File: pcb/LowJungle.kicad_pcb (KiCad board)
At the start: 2 copper layers, 378.6 x 152.4 mm, 255 parts

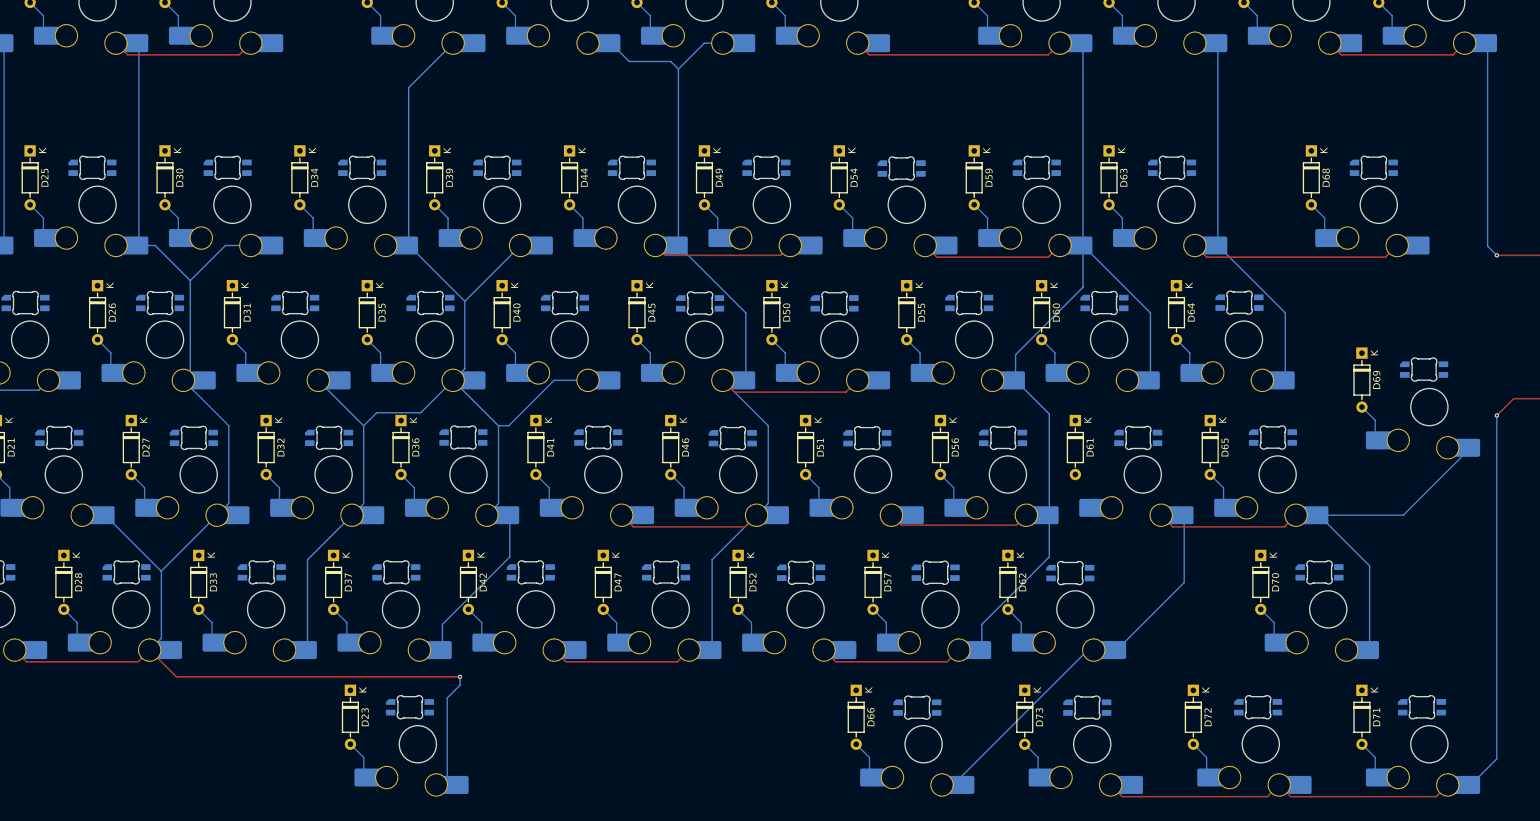
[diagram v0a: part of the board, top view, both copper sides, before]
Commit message: Added stabilizers
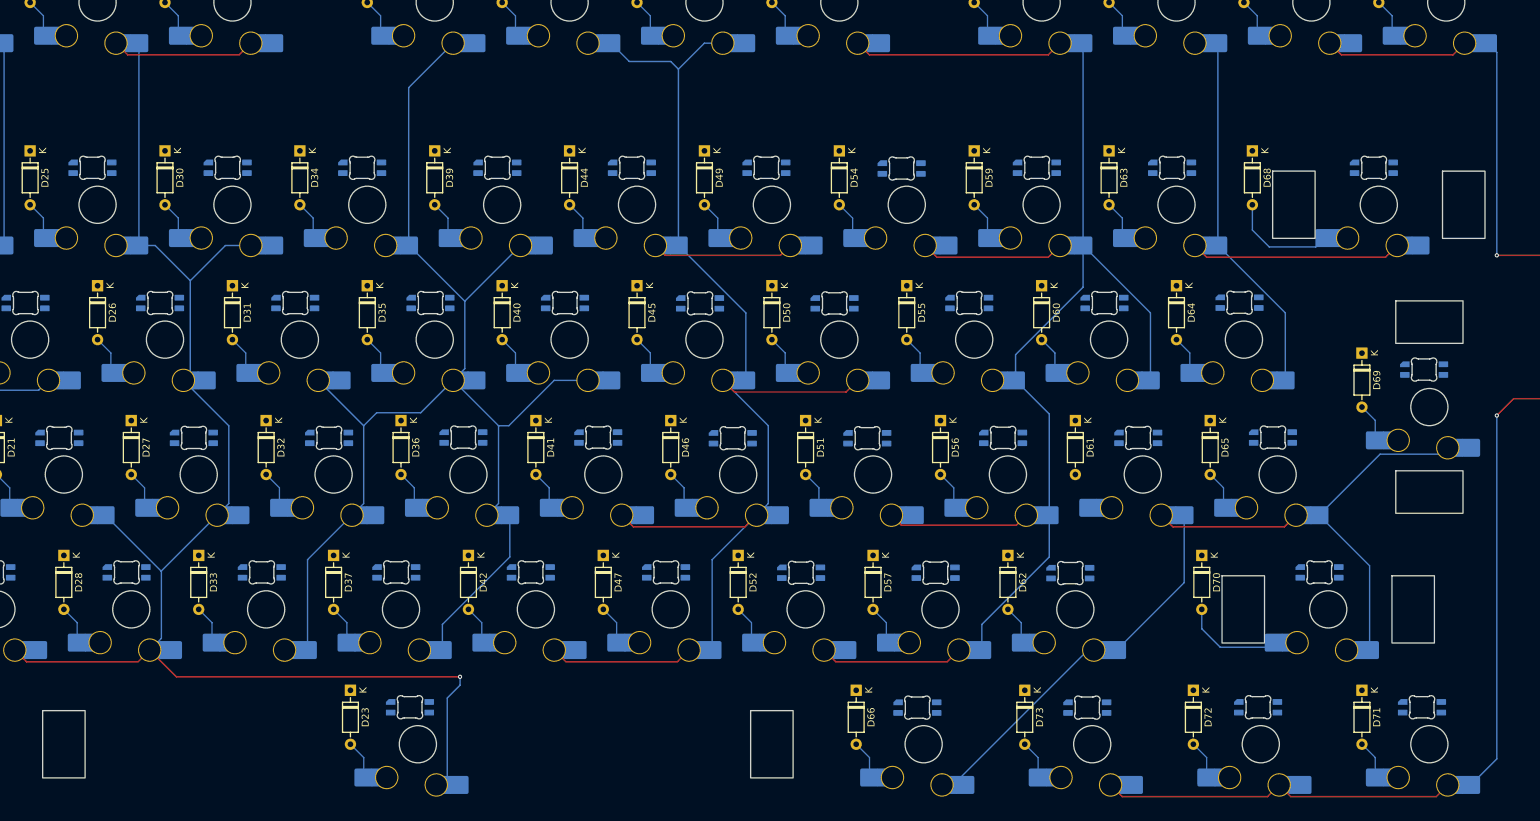
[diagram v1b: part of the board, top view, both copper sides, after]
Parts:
- moved D68 8.33 mm to (277.4, 59.1)
- moved D70 8.33 mm to (270.3, 116.2)
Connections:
- LED1 pad 3: Net-(LED1-DIN) -> /LEDs/DIN
- LED18 pad 3: Net-(LED1-DOUT) -> Net-(LED18-DIN)
- LED2 pad 2: Net-(LED1-DIN) -> Net-(LED2-DOUT)
- LED2 pad 3: Net-(LED2-DIN) -> Net-(LED1-DOUT)
- LED3 pad 2: Net-(LED2-DIN) -> Net-(LED3-DOUT)
- LED3 pad 3: Net-(LED3-DIN) -> Net-(LED2-DOUT)
- LED4 pad 2: Net-(LED3-DIN) -> Net-(LED4-DOUT)
- LED4 pad 3: Net-(LED4-DIN) -> Net-(LED3-DOUT)
- LED5 pad 2: Net-(LED4-DIN) -> Net-(LED5-DOUT)
- LED5 pad 3: Net-(LED5-DIN) -> Net-(LED4-DOUT)
- LED55 pad 2: Net-(LED55-DOUT) -> unconnected-(LED55-DOUT-Pad2)
- LED56 pad 2: Net-(LED55-DIN) -> Net-(LED56-DOUT)
- LED6 pad 2: Net-(LED5-DIN) -> Net-(LED6-DOUT)
- LED6 pad 3: Net-(LED6-DIN) -> Net-(LED5-DOUT)
- LED7 pad 2: Net-(LED6-DIN) -> Net-(LED7-DOUT)
- LED7 pad 3: Net-(LED7-DIN) -> Net-(LED6-DOUT)
- LED72 pad 3: Net-(LED55-DOUT) -> Net-(LED56-DOUT)
- LED8 pad 2: Net-(LED7-DIN) -> Net-(LED8-DOUT)
- LED8 pad 3: Net-(LED8-DIN) -> Net-(LED7-DOUT)
- LED82 pad 2: unconnected-(LED82-DOUT-Pad2) -> Net-(LED55-DIN)
- LED9 pad 2: Net-(LED8-DIN) -> Net-(LED18-DIN)
- LED9 pad 3: /LEDs/DIN -> Net-(LED8-DOUT)
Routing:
- net Net-(D68-A): track 5.48 -> 15.3 mm
- net Net-(D70-A): track 5.48 -> 14.3 mm
- net /KeyMatrix/COLUM_7: track 203.3 -> 200.1 mm
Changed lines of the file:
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@@
 	(net 107 "Net-(LED1-DOUT)")
 	(net 108 "VBUS")
-	(net 109 "Net-(LED1-DIN)")
-	(net 110 "Net-(LED2-DIN)")
-	(net 111 "Net-(LED3-DIN)")
-	(net 112 "Net-(LED4-DIN)")
-	(net 113 "Net-(LED5-DIN)")
-	(net 114 "Net-(LED6-DIN)")
-	(net 115 "Net-(LED7-DIN)")
-	(net 116 "Net-(LED8-DIN)")
+	(net 109 "Net-(LED2-DOUT)")
+	(net 110 "Net-(LED3-DOUT)")
+	(net 111 "Net-(LED4-DOUT)")
+	(net 112 "Net-(LED5-DOUT)")
+	(net 113 "Net-(LED6-DOUT)")
+	(net 114 "Net-(LED7-DOUT)")
+	(net 115 "Net-(LED8-DOUT)")
+	(net 116 "Net-(LED18-DIN)")
 	(net 117 "/LEDs/DIN")
 	(net 118 "Net-(LED10-DOUT)")
@@
 	(net 161 "Net-(LED52-DIN)")
 	(net 162 "Net-(LED53-DIN)")
-	(net 163 "Net-(LED55-DOUT)")
+	(net 163 "unconnected-(LED55-DOUT-Pad2)")
 	(net 164 "Net-(LED55-DIN)")
 	(net 165 "Net-(LED56-DIN)")
@@
 	(net 189 "Net-(LED80-DIN)")
 	(net 190 "Net-(LED82-DIN)")
-	(net 191 "unconnected-(LED82-DOUT-Pad2)")
+	(net 191 "Net-(LED56-DOUT)")
 	(net 192 "Net-(LED83-DIN)")
 	(net 193 "Net-(LED84-DIN)")
@@
 			(layer "Eco2.User")
 		)
+		(fp_rect
+			(start -15 -4.7625)
+			(end -9 4.7375)
+			(stroke
+				(width 0.05)
+				(type solid)
+			)
+			(fill no)
+			(layer "Edge.Cuts")
+		)
+		(fp_rect
+			(start 9 -4.75)
+			(end 15 4.75)
+			(stroke
+				(width 0.05)
+				(type solid)
+			)
+			(fill no)
+			(layer "Edge.Cuts")
+		)
 		(fp_line
 			(start -9.045 3.4)
@@
 	(footprint "Diode_THT:D_DO-35_SOD27_P7.62mm_Horizontal"
 		(layer "F.Cu")
-		(at 285.75 59.055 -90)
+		(at 277.415625 59.055 -90)
 		(descr "Diode, DO-35_SOD27 series, Axial, Horizontal, pin pitch=7.62mm, , length*diameter=4*2mm^2, , http://www.diodes.com/_files/packages/DO-35.pdf")
 		(tags "Diode DO-35_SOD27 series Axial Horizontal pin pitch 7.62mm  length 4mm diameter 2mm")
@@
 			(layer "Eco2.User")
 		)
+		(fp_rect
+			(start -4.75 -15)
+			(end 4.75 -9)
+			(stroke
+				(width 0.05)
+				(type solid)
+			)
+			(fill no)
+			(layer "Edge.Cuts")
+		)
+		(fp_rect
+			(start -4.75 9)
+			(end 4.75 15)
+			(stroke
+				(width 0.05)
+				(type solid)
+			)
+			(fill no)
+			(layer "Edge.Cuts")
+		)
 		(fp_line
 			(start -9.045 3.4)
@@
 			(layer "Eco2.User")
 		)
+		(fp_rect
+			(start -15 -4.75)
+			(end -9 4.75)
+			(stroke
+				(width 0.05)
+				(type solid)
+			)
+			(fill no)
+			(layer "Edge.Cuts")
+		)
+		(fp_rect
+			(start 9 -4.75)
+			(end 15 4.75)
+			(stroke
+				(width 0.05)
+				(type solid)
+			)
+			(fill no)
+			(layer "Edge.Cuts")
+		)
 		(fp_line
 			(start -9.045 3.4)
@@
 	(footprint "Diode_THT:D_DO-35_SOD27_P7.62mm_Horizontal"
 		(layer "F.Cu")
-		(at 278.60625 116.205 -90)
+		(at 270.271875 116.205 -90)
 		(descr "Diode, DO-35_SOD27 series, Axial, Horizontal, pin pitch=7.62mm, , length*diameter=4*2mm^2, , http://www.diodes.com/_files/packages/DO-35.pdf")
 		(tags "Diode DO-35_SOD27 series Axial Horizontal pin pitch 7.62mm  length 4mm diameter 2mm")
@@
 			(layer "Eco2.User")
 		)
+		(fp_rect
+			(start -53 -4.75)
+			(end -47 4.75)
+			(stroke
+				(width 0.05)
+				(type solid)
+			)
+			(fill no)
+			(layer "Edge.Cuts")
+		)
+		(fp_rect
+			(start 47 -4.75)
+			(end 53 4.75)
+			(stroke
+				(width 0.05)
+				(type solid)
+			)
+			(fill no)
+			(layer "Edge.Cuts")
+		)
 		(fp_line
 			(start -9.045 3.4)
@@
 			(layers "B.Cu" "B.Mask" "B.Paste")
 			(roundrect_rratio 0.1)
-			(net 113 "Net-(LED5-DIN)")
+			(net 113 "Net-(LED6-DOUT)")
 			(pinfunction "DOUT")
 			(pintype "output")
@@
 			(layers "B.Cu" "B.Mask" "B.Paste")
 			(roundrect_rratio 0.1)
-			(net 114 "Net-(LED6-DIN)")
+			(net 112 "Net-(LED5-DOUT)")
 			(pinfunction "DIN")
 			(pintype "input")
@@
 			(layers "B.Cu" "B.Mask" "B.Paste")
 			(roundrect_rratio 0.1)
-			(net 107 "Net-(LED1-DOUT)")
+			(net 116 "Net-(LED18-DIN)")
 			(pinfunction "DIN")
 			(pintype "input")
@@
 			(layers "B.Cu" "B.Mask" "B.Paste")
 			(roundrect_rratio 0.1)
-			(net 109 "Net-(LED1-DIN)")
+			(net 109 "Net-(LED2-DOUT)")
 			(pinfunction "DOUT")
 			(pintype "output")
@@
 			(layers "B.Cu" "B.Mask" "B.Paste")
 			(roundrect_rratio 0.1)
-			(net 110 "Net-(LED2-DIN)")
+			(net 107 "Net-(LED1-DOUT)")
 			(pinfunction "DIN")
 			(pintype "input")
@@
 			(layers "B.Cu" "B.Mask" "B.Paste")
 			(roundrect_rratio 0.1)
-			(net 111 "Net-(LED3-DIN)")
+			(net 111 "Net-(LED4-DOUT)")
 			(pinfunction "DOUT")
 			(pintype "output")
@@
 			(layers "B.Cu" "B.Mask" "B.Paste")
 			(roundrect_rratio 0.1)
-			(net 112 "Net-(LED4-DIN)")
+			(net 110 "Net-(LED3-DOUT)")
 			(pinfunction "DIN")
 			(pintype "input")
@@
 			(layers "B.Cu" "B.Mask" "B.Paste")
 			(roundrect_rratio 0.1)
-			(net 191 "unconnected-(LED82-DOUT-Pad2)")
+			(net 164 "Net-(LED55-DIN)")
 			(pinfunction "DOUT")
-			(pintype "output+no_connect")
+			(pintype "output")
 		)
 		(pad "3" smd roundrect
@@
 			(layers "B.Cu" "B.Mask" "B.Paste")
 			(roundrect_rratio 0.1)
-			(net 109 "Net-(LED1-DIN)")
+			(net 117 "/LEDs/DIN")
 			(pinfunction "DIN")
 			(pintype "input")
@@
 			(layers "B.Cu" "B.Mask" "B.Paste")
 			(roundrect_rratio 0.1)
-			(net 114 "Net-(LED6-DIN)")
+			(net 114 "Net-(LED7-DOUT)")
 			(pinfunction "DOUT")
 			(pintype "output")
@@
 			(layers "B.Cu" "B.Mask" "B.Paste")
 			(roundrect_rratio 0.1)
-			(net 115 "Net-(LED7-DIN)")
+			(net 113 "Net-(LED6-DOUT)")
 			(pinfunction "DIN")
 			(pintype "input")
@@
 			(layers "B.Cu" "B.Mask" "B.Paste")
 			(roundrect_rratio 0.1)
-			(net 112 "Net-(LED4-DIN)")
+			(net 112 "Net-(LED5-DOUT)")
 			(pinfunction "DOUT")
 			(pintype "output")
@@
 			(layers "B.Cu" "B.Mask" "B.Paste")
 			(roundrect_rratio 0.1)
-			(net 113 "Net-(LED5-DIN)")
+			(net 111 "Net-(LED4-DOUT)")
 			(pinfunction "DIN")
 			(pintype "input")
@@
 			(layers "B.Cu" "B.Mask" "B.Paste")
 			(roundrect_rratio 0.1)
-			(net 116 "Net-(LED8-DIN)")
+			(net 116 "Net-(LED18-DIN)")
 			(pinfunction "DOUT")
 			(pintype "output")
@@
 			(layers "B.Cu" "B.Mask" "B.Paste")
 			(roundrect_rratio 0.1)
-			(net 117 "/LEDs/DIN")
+			(net 115 "Net-(LED8-DOUT)")
 			(pinfunction "DIN")
 			(pintype "input")
@@
 			(layers "B.Cu" "B.Mask" "B.Paste")
 			(roundrect_rratio 0.1)
-			(net 110 "Net-(LED2-DIN)")
+			(net 110 "Net-(LED3-DOUT)")
 			(pinfunction "DOUT")
 			(pintype "output")
@@
 			(layers "B.Cu" "B.Mask" "B.Paste")
 			(roundrect_rratio 0.1)
-			(net 111 "Net-(LED3-DIN)")
+			(net 109 "Net-(LED2-DOUT)")
 			(pinfunction "DIN")
 			(pintype "input")
@@
 			(layers "B.Cu" "B.Mask" "B.Paste")
 			(roundrect_rratio 0.1)
-			(net 163 "Net-(LED55-DOUT)")
+			(net 163 "unconnected-(LED55-DOUT-Pad2)")
 			(pinfunction "DOUT")
-			(pintype "output")
+			(pintype "output+no_connect")
 		)
 		(pad "3" smd roundrect
@@
 			(layers "B.Cu" "B.Mask" "B.Paste")
 			(roundrect_rratio 0.1)
-			(net 163 "Net-(LED55-DOUT)")
+			(net 191 "Net-(LED56-DOUT)")
 			(pinfunction "DIN")
 			(pintype "input")
@@
 			(layers "B.Cu" "B.Mask" "B.Paste")
 			(roundrect_rratio 0.1)
-			(net 115 "Net-(LED7-DIN)")
+			(net 115 "Net-(LED8-DOUT)")
 			(pinfunction "DOUT")
 			(pintype "output")
@@
 			(layers "B.Cu" "B.Mask" "B.Paste")
 			(roundrect_rratio 0.1)
-			(net 116 "Net-(LED8-DIN)")
+			(net 114 "Net-(LED7-DOUT)")
 			(pinfunction "DIN")
 			(pintype "input")
@@
 			(layers "B.Cu" "B.Mask" "B.Paste")
 			(roundrect_rratio 0.1)
-			(net 164 "Net-(LED55-DIN)")
+			(net 191 "Net-(LED56-DOUT)")
 			(pinfunction "DOUT")
 			(pintype "output")
@@
 	)
 	(segment
-		(start 298.73875 110.525)
-		(end 286.8325 110.525)
-		(width 0.2)
-		(layer "B.Cu")
-		(net 67)
-	)
-	(segment
 		(start 272.545 43.85)
 		(end 272.545 72.425)
@@
 	)
 	(segment
+		(start 286.8325 110.525)
+		(end 295.4565 101.901)
+		(width 0.2)
+		(layer "B.Cu")
+		(net 67)
+	)
+	(segment
 		(start 293.97625 129.575)
 		(end 293.97625 117.66875)
@@
 	)
 	(segment
+		(start 295.4565 101.901)
+		(end 304.11775 101.901)
+		(width 0.2)
+		(layer "B.Cu")
+		(net 67)
+	)
+	(segment
 		(start 267.7825 120.05)
 		(end 258.2575 129.575)
@@
 	)
 	(segment
-		(start 308.26375 101)
-		(end 298.73875 110.525)
+		(start 272.545 72.425)
+		(end 282.07 81.95)
 		(width 0.2)
 		(layer "B.Cu")
@@
 	)
 	(segment
-		(start 272.545 72.425)
-		(end 282.07 81.95)
+		(start 304.11775 101.901)
+		(end 305.01875 101)
 		(width 0.2)
 		(layer "B.Cu")
@@
 	)
 	(segment
+		(start 286.376875 72.628125)
+		(end 279.796875 72.628125)
+		(width 0.2)
+		(layer "B.Cu")
+		(net 75)
+	)
+	(segment
 		(start 287.63 71.375)
-		(end 287.63 68.555)
-		(width 0.175)
+		(end 286.376875 72.628125)
+		(width 0.2)
 		(layer "B.Cu")
 		(net 75)
 	)
 	(segment
-		(start 287.63 68.555)
-		(end 285.75 66.675)
-		(width 0.175)
+		(start 277.415625 70.246875)
+		(end 277.415625 66.675)
+		(width 0.2)
+		(layer "B.Cu")
+		(net 75)
+	)
+	(segment
+		(start 279.796875 72.628125)
+		(end 277.415625 70.246875)
+		(width 0.2)
 		(layer "B.Cu")
 		(net 75)
@@
 	)
 	(segment
-		(start 280.48625 125.705)
-		(end 278.60625 123.825)
-		(width 0.175)
+		(start 272.882308 129.176)
+		(end 279.83525 129.176)
+		(width 0.2)
 		(layer "B.Cu")
 		(net 77)
 	)
 	(segment
-		(start 280.48625 128.525)
-		(end 280.48625 125.705)
-		(width 0.175)
+		(start 270.271875 123.825)
+		(end 270.271875 126.565567)
+		(width 0.2)
+		(layer "B.Cu")
+		(net 77)
+	)
+	(segment
+		(start 270.271875 126.565567)
+		(end 272.882308 129.176)
+		(width 0.2)
+		(layer "B.Cu")
+		(net 77)
+	)
+	(segment
+		(start 279.83525 129.176)
+		(end 280.48625 128.525)
+		(width 0.2)
 		(layer "B.Cu")
 		(net 77)
@@
 	)
 	(segment
-		(start 310.645 72.52)
+		(start 311.94375 45.14875)
 		(end 311.94375 73.81875)
 		(width 0.2)
@@
 	)
 	(segment
-		(start 310.645 43.85)
-		(end 310.645 72.52)
-		(width 0.2)
-		(layer "B.Cu")
-		(net 79)
-	)
-	(segment
 		(start 311.94375 144.945)
 		(end 311.94375 96.440625)
@@
 		(width 0.2)
 		(layer "B.Cu")
+		(net 79)
+	)
+	(segment
+		(start 310.645 43.85)
+		(end 311.94375 45.14875)
+		(width 0.2)
+		(layer "B.Cu")
